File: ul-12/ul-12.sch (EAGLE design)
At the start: 39 parts, among them IC1 24C64SM, IC2 CY7C68013-56PVC, IC3 LD1117, IC4 24C64SM, IC5 24C64P, Q2 24 MHz, X1 USB-MINIB-BUV2, X2 F25D, X3 F25D

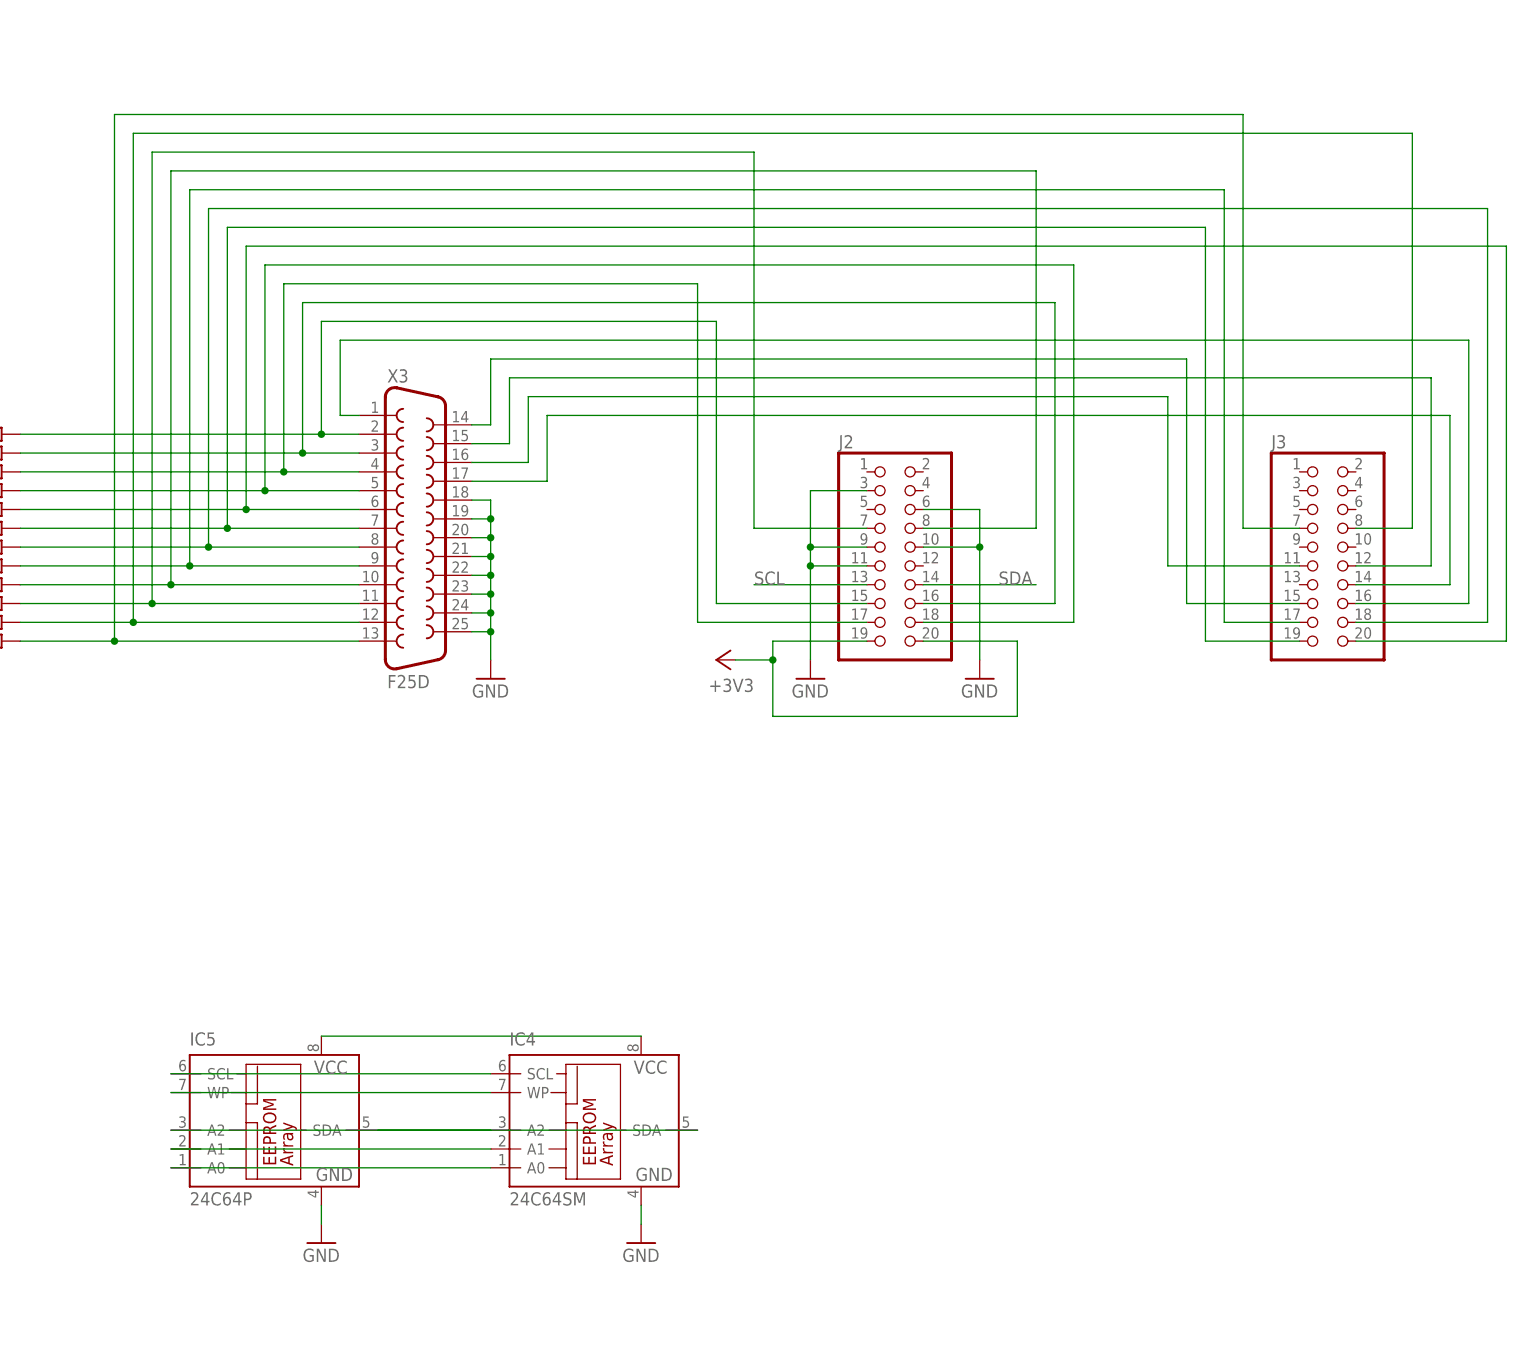
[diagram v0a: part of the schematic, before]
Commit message: .
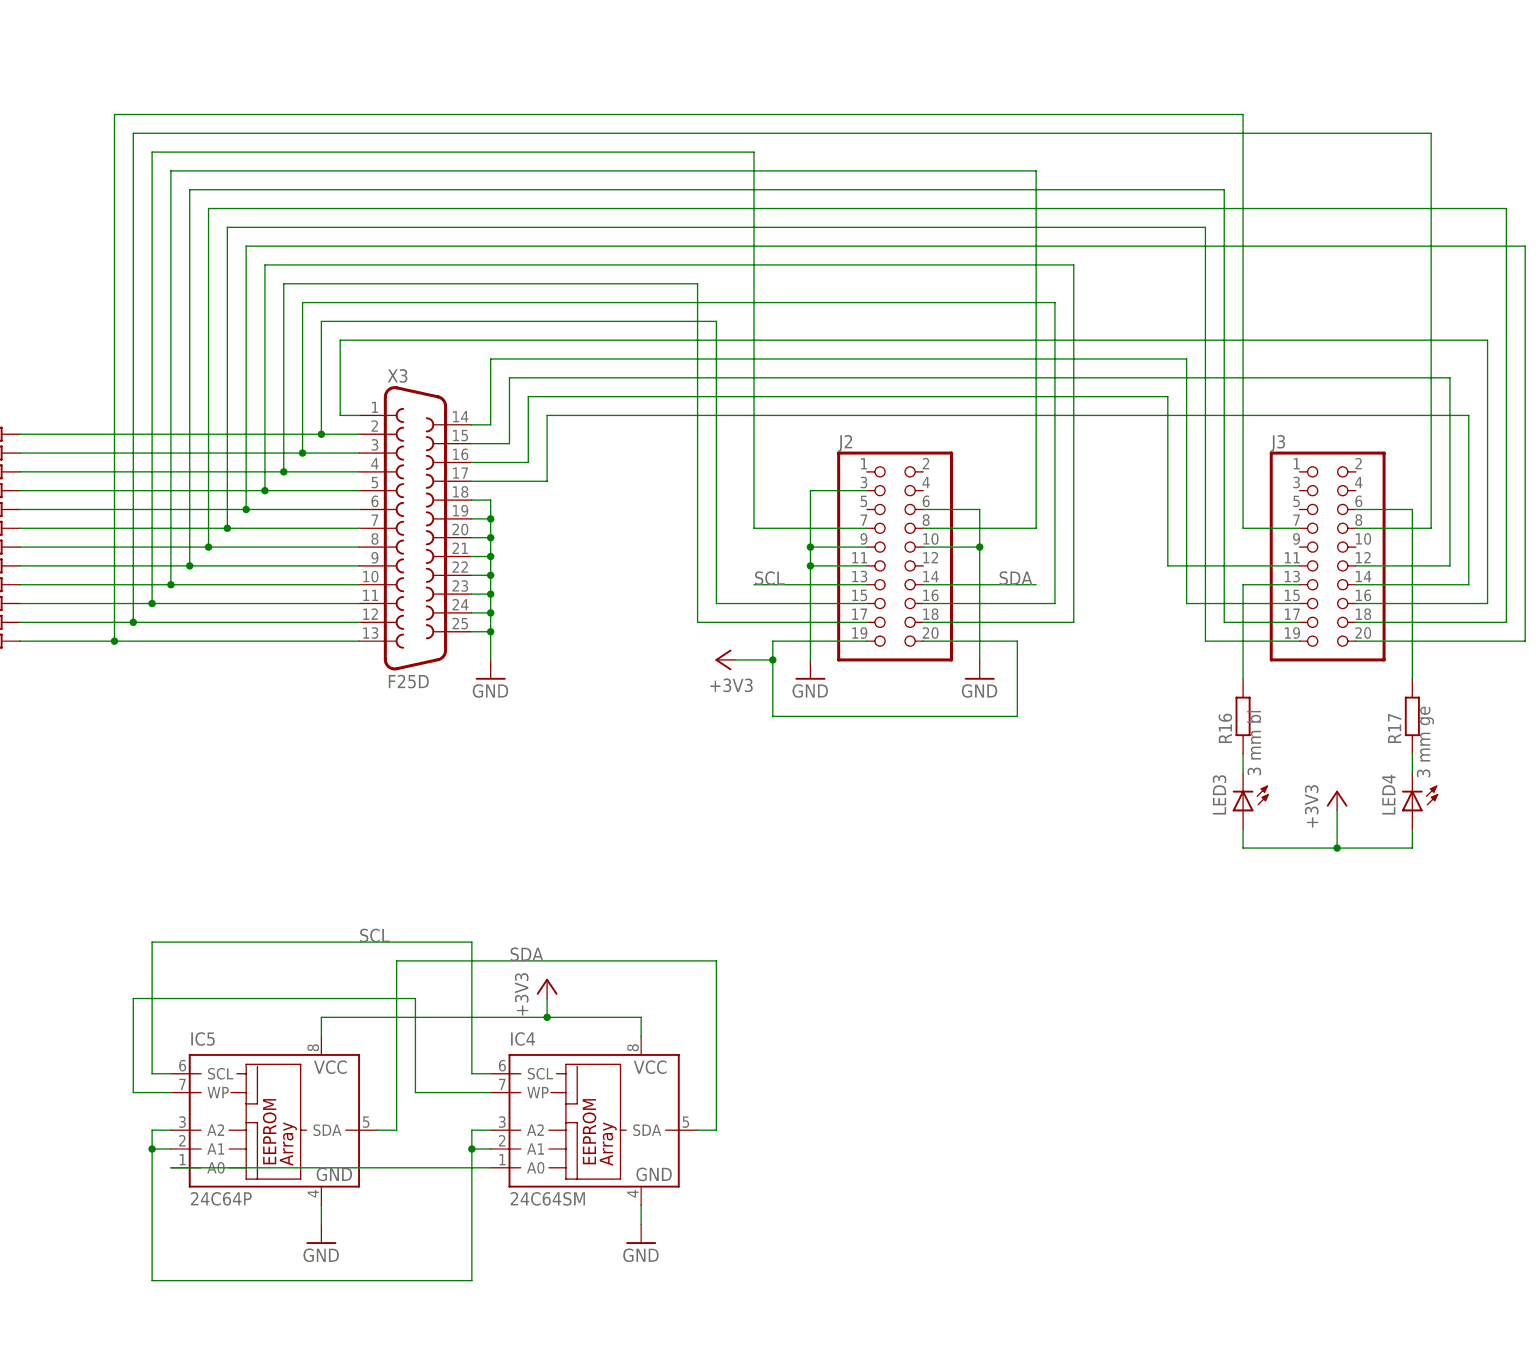
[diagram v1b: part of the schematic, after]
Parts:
- added LED3: 3 mm bl, led:LED3MM
- added LED4: 3 mm ge, led:LED3MM
- added R16, R17: (no value), rcl:R-EU_R0805
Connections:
- removed net N$45: IC4.VCC, IC5.VCC
- removed net N$47: IC4.SCL, IC5.SCL
- removed net N$48: IC4.SDA, IC5.SDA
- removed net N$51: IC4.A2, IC5.A2
- new net N$25: J3.13, R16.2
- new net N$26: LED3.C, R16.1
- new net N$27: J3.6, R17.2
- new net N$28: LED4.C, R17.1
- net +3V3: now also IC4.VCC, IC5.VCC, LED3.A, LED4.A
- net N$50: now also IC4.A2, IC5.A2
- net SCL: now also IC4.SCL, IC5.SCL
- net SDA: now also IC4.SDA, IC5.SDA
